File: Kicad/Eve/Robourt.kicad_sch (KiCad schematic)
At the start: 77 parts, among them IC101 STM32U535RET6, J1 Conn_02x08_Odd_Even, J102 Conn_01x02, J103 Conn_01x02, J108 Conn_01x03, J109 Conn_01x03, J110 Conn_01x02, Q101 NMOS, Y101 Crystal

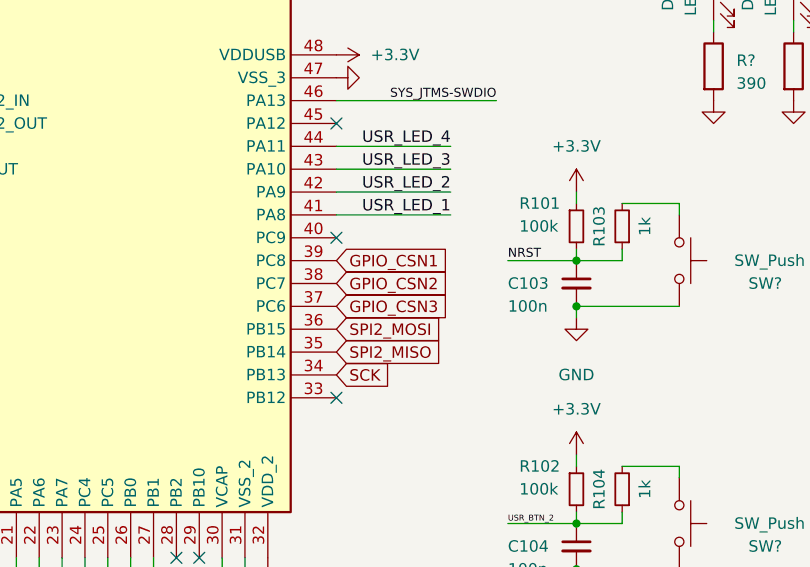
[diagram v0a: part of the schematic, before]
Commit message: update
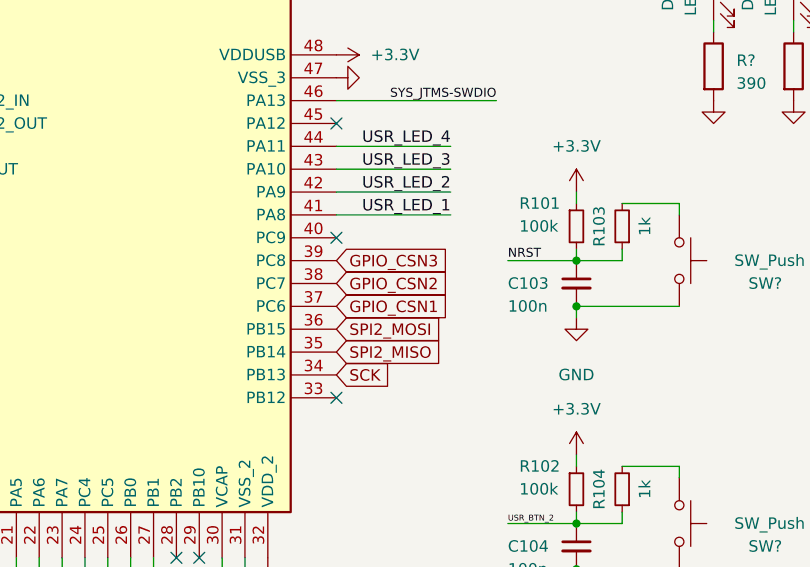
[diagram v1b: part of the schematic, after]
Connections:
- net GPIO_CSN1: now also IC101.37 (PC6); no longer IC101.39 (PC8)
- net GPIO_CSN3: now also IC101.39 (PC8); no longer IC101.37 (PC6)
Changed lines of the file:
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@@
+    )
+  )
+  (global_label "GPIO_CSN3" (shape input) (at 96.52 135.89 0) (fields_autoplaced)
+    (effects (font (size 1.27 1.27)) (justify left))
+    (property "Intersheetrefs" "${INTERSHEET_REFS}" (at 109.8882 135.89 0)
+      (effects (font (size 1.27 1.27)) (justify left) hide)
     )
   )
@@
     )
   )
+  (global_label "GPIO_CSN1" (shape input) (at 96.52 140.97 0) (fields_autoplaced)
+    (effects (font (size 1.27 1.27)) (justify left))
+    (property "Intersheetrefs" "${INTERSHEET_REFS}" (at 109.8882 140.97 0)
+      (effects (font (size 1.27 1.27)) (justify left) hide)
+    )
+  )
   (global_label "GND7" (shape input) (at 266.7 241.3 0) (fields_autoplaced)
     (effects (font (size 1.27 1.27)) (justify left))
@@
     )
   )
-  (global_label "GPIO_CSN1" (shape input) (at 96.52 135.89 0) (fields_autoplaced)
-    (effects (font (size 1.27 1.27)) (justify left))
-    (property "Intersheetrefs" "${INTERSHEET_REFS}" (at 109.8882 135.89 0)
-      (effects (font (size 1.27 1.27)) (justify left) hide)
-    )
-  )
   (global_label "UART4_RX" (shape input) (at 96.52 250.19 180) (fields_autoplaced)
     (effects (font (size 1.27 1.27)) (justify right))
@@
       (effects (font (size 1.27 1.27)) (justify left) hide)
     )
-  )
-  (global_label "GPIO_CSN3" (shape input) (at 96.52 140.97 0) (fields_autoplaced)
-    (effects (font (size 1.27 1.27)) (justify left))
-    (property "Intersheetrefs" "${INTERSHEET_REFS}" (at 109.8882 140.97 0)
-      (effects (font (size 1.27 1.27)) (justify left) hide)
-    )
